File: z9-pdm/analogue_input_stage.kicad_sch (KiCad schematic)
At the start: 7 parts

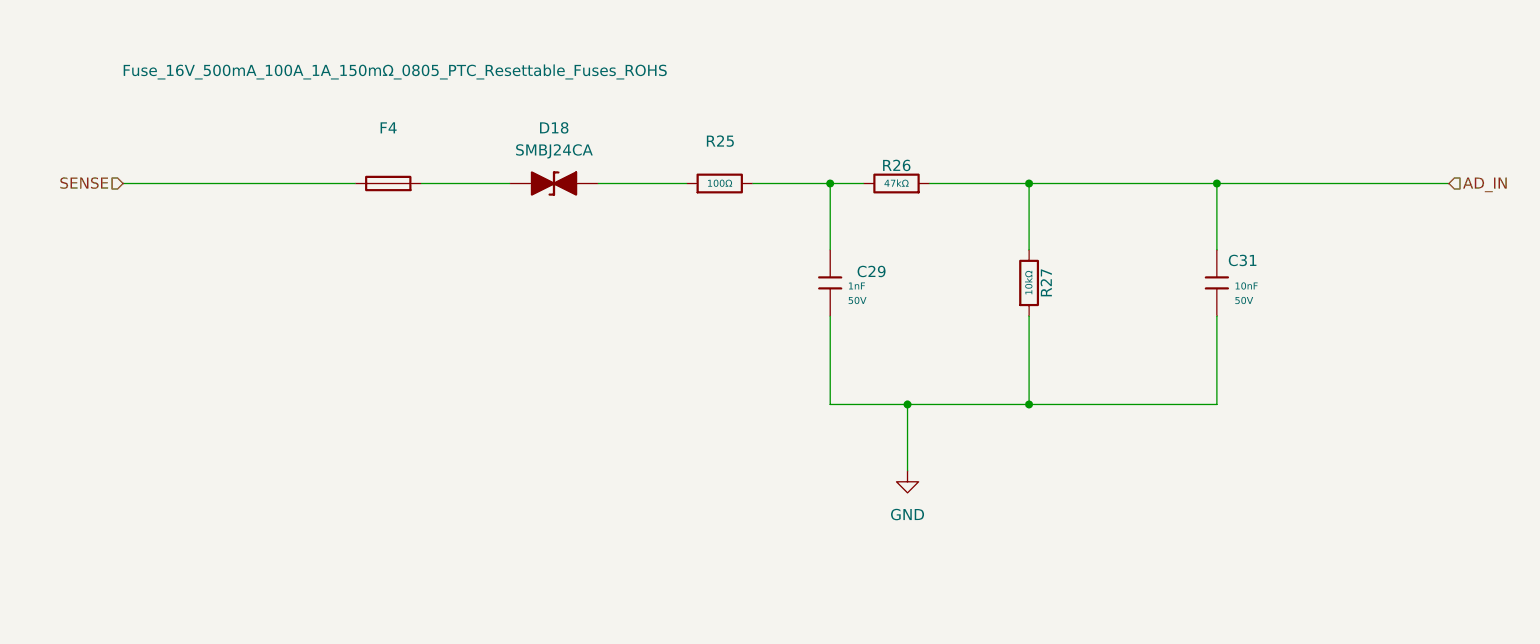
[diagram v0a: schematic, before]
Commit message: pre replicate analogue chans
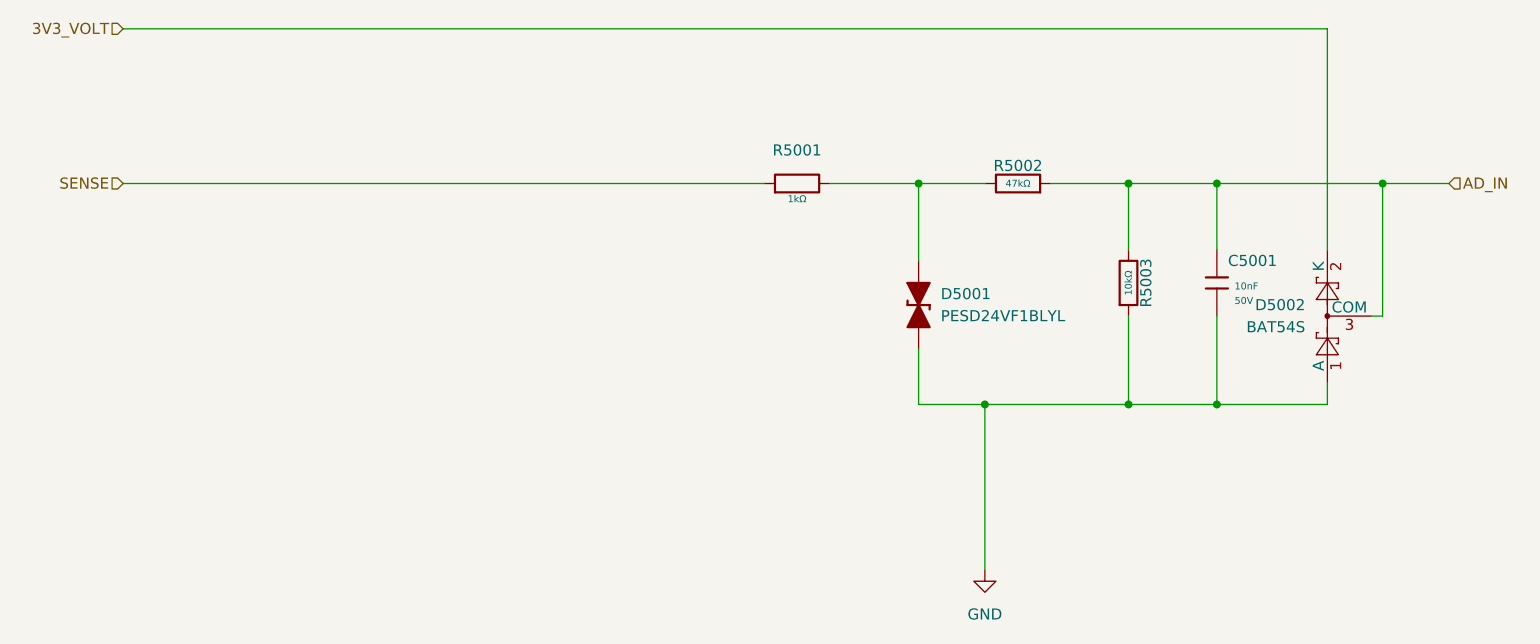
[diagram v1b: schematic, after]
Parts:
- removed C29: 1nF, PCM_JLCPCB:C_0603, symbol PCM_JLCPCB-Capacitors:0603,1nF
- removed D18: SMBJ24CA, PCM_Diode_SMD_AKL:D_SMB_TVS, symbol PCM_Diode_TVS_AKL:SMBJ24CA
- removed F4: Fuse_16V_500mA_100A_1A_150mΩ_0805_PTC_Resettable_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, Fuse:Fuse_0805_2012Metric, symbol dnt_global:Fuse_16V_500mA_100A_1A_150mΩ_0805_PTC_Resettable_Fuses_ROHS
- removed R25: 100Ω, PCM_JLCPCB:R_0603, symbol PCM_JLCPCB-Resistors:0603,100Ω
- added D5001: PESD24VF1BLYL, PCM_Diode_SMD_AKL:D_SOD-323_TVS, symbol PCM_Diode_TVS_AKL:PESD24VL1BA
- added D5002: BAT54S, Package_TO_SOT_SMD:SOT-23, symbol Diode:BAT54S
- added R5001: 1kΩ, PCM_JLCPCB:R_0805, symbol PCM_JLCPCB-Resistors:0805,1kΩ
- renumbered C31 to C5001, R26 to R5002, R27 to R5003
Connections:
- net AD_IN: now also D5002.3 (COM)
- net GND: now also D5001.1 (K), D5002.1 (A)
- net SENSE: now also R5001.1
- net at R5002.2: now also D5001.2 (A), R5001.2
- new net 3V3_VOLT: D5002.2 (K)
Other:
- moved on the sheet: R5002, R5003
